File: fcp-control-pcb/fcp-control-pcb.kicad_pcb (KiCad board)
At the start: 2 copper layers, 136 x 104.8 mm, 97 parts, among them IC1 L01Z050S05, J1 Conn_01x15_Female, J10 LittlePump, J11 BigPump, J12 OUT0, J13 Conn_01x10_Male, J14 Conn_01x10_Male, J15 Conn_01x10_Male, J16 ExtraAnalogs, J2 Conn_01x15_Female, J3 CAPACITOR, J4 FUELCELL, J5 ArduinoVCCPower, J6 DISCHARGER, J7 CHARGER, J8 LimiterBypass, J9 Current_Mode, Q1 AONR21321, Q2 Q_NMOS_GDS, Q3 Q_NMOS_GDS, Q4 Q_NMOS_GDS, U1 MAX15462AB, U10 ADC1283, U2 LM311DR, U3 TLI4971-A050T5-U-E0001, U4 AS78L05RTR-G1, U5 ZXGD3003E6, U6 AS78L05RTR-G1, U7 ADC1283, U8 ADC1283, U9 ADC1283

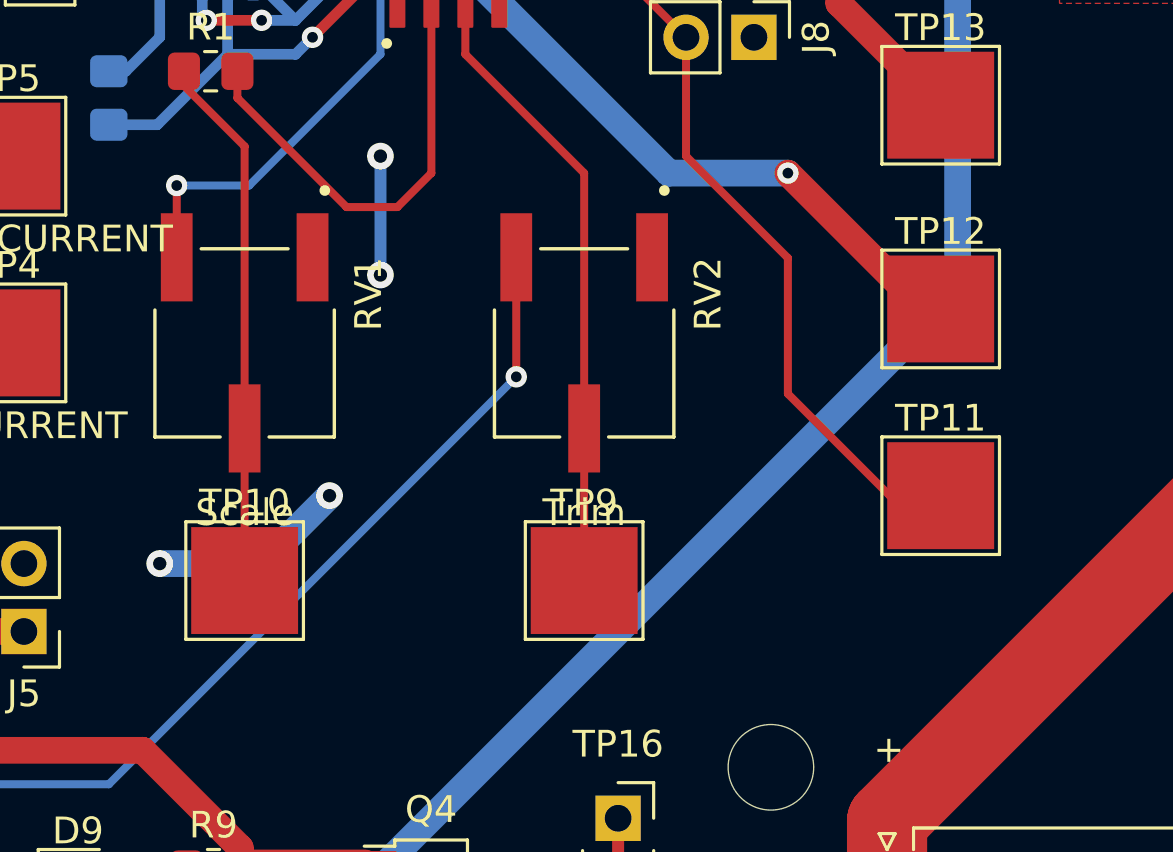
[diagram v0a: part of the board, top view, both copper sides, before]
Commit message: label tps
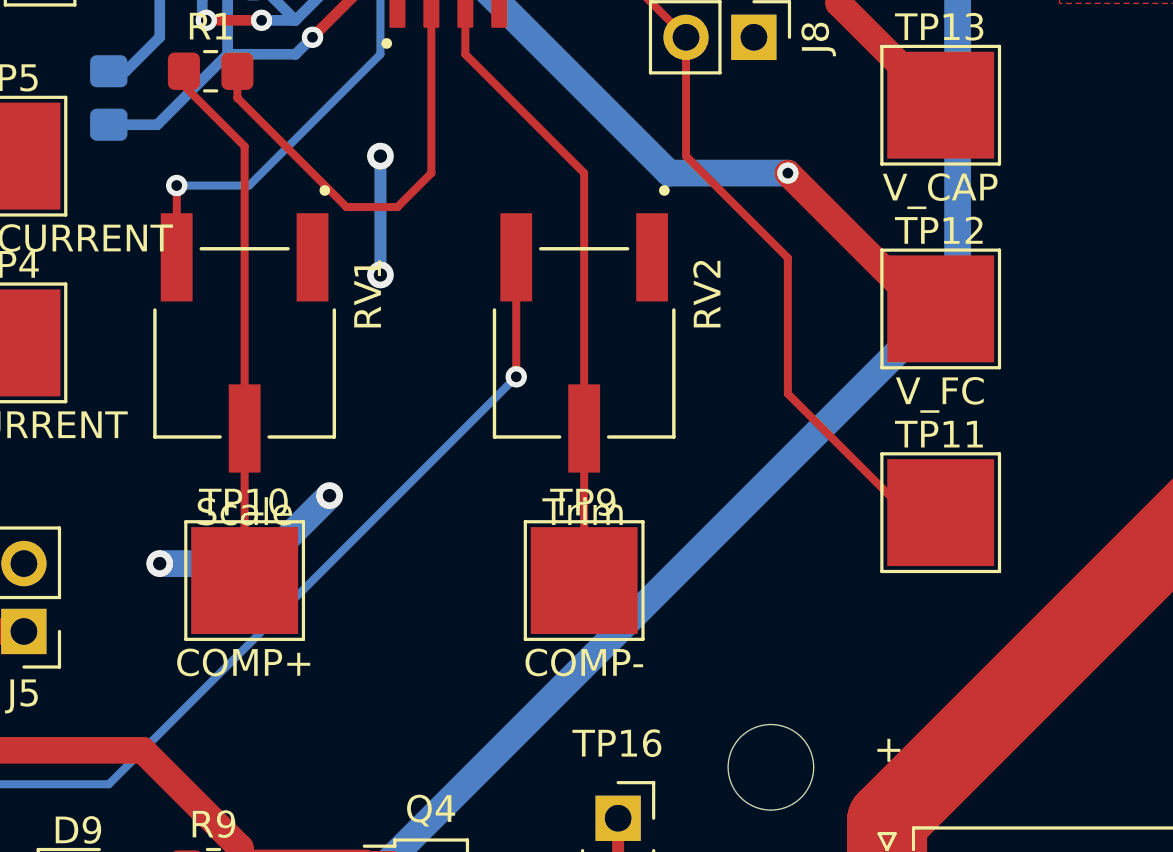
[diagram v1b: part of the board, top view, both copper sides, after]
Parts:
- moved TP11 0.64 mm to (183.5, 94.0)
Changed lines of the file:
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@@
   )
   (footprint "TestPoint:TestPoint_Pad_4.0x4.0mm" (layer "F.Cu")
-    (at 183.515 93.345)
+    (at 183.515 93.98)
     (descr "SMD rectangular pad as test Point, square 4.0mm side length")
     (tags "test point SMD pad rectangle square")
@@
       (effects (font (size 1 1) (thickness 0.15)))
     )
-    (fp_text value "COMP+" (at 0 3.1) (layer "F.Fab")
+    (fp_text value "COMP+" (at 0 3.1) (layer "F.SilkS")
       (effects (font (size 1 1) (thickness 0.15)))
     )
@@
       (effects (font (size 1 1) (thickness 0.15)))
     )
-    (fp_text value "V_FC" (at 0 3.1) (layer "F.Fab")
+    (fp_text value "V_FC" (at 0 3.1) (layer "F.SilkS")
       (effects (font (size 1 1) (thickness 0.15)))
     )
@@
       (effects (font (size 1 1) (thickness 0.15)))
     )
-    (fp_text value "COMP-" (at 0 3.1) (layer "F.Fab")
+    (fp_text value "COMP-" (at 0 3.1) (layer "F.SilkS")
       (effects (font (size 1 1) (thickness 0.15)))
     )
@@
       (effects (font (size 1 1) (thickness 0.15)))
     )
-    (fp_text value "V_CAP" (at 0 3.1) (layer "F.Fab")
+    (fp_text value "V_CAP" (at 0 3.1) (layer "F.SilkS")
       (effects (font (size 1 1) (thickness 0.15)))
     )
